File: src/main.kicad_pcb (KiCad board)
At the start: 4 copper layers, 54 parts, among them P301 CONN_01X15, P302 CONN_01X03, P501 CONN_01X07, Q501 MMBT3904, Q502 MMBT3904, U301 LM741, U302 DG444, U303 LM741, U304 LM741, U305 LM311N, U501 LM741, U502 LM741, U503 2DW232

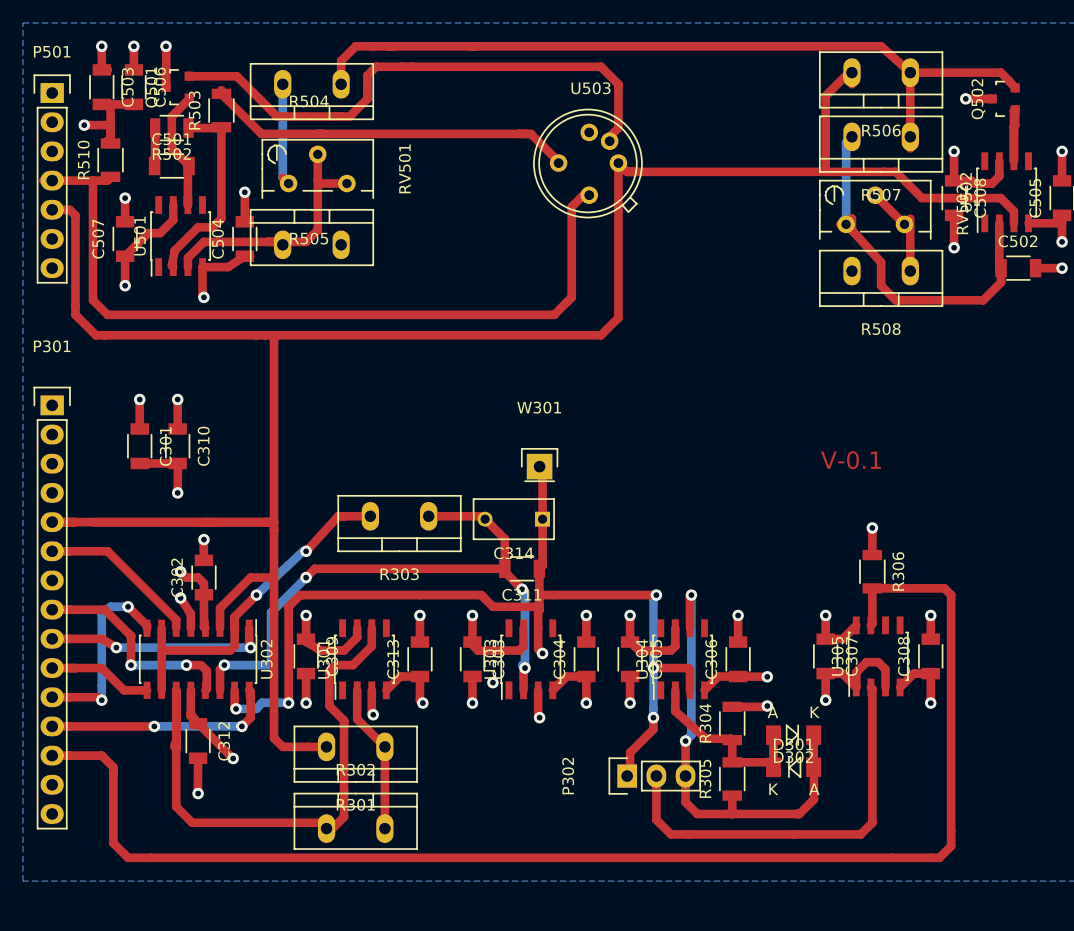
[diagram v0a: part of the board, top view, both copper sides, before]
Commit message: update
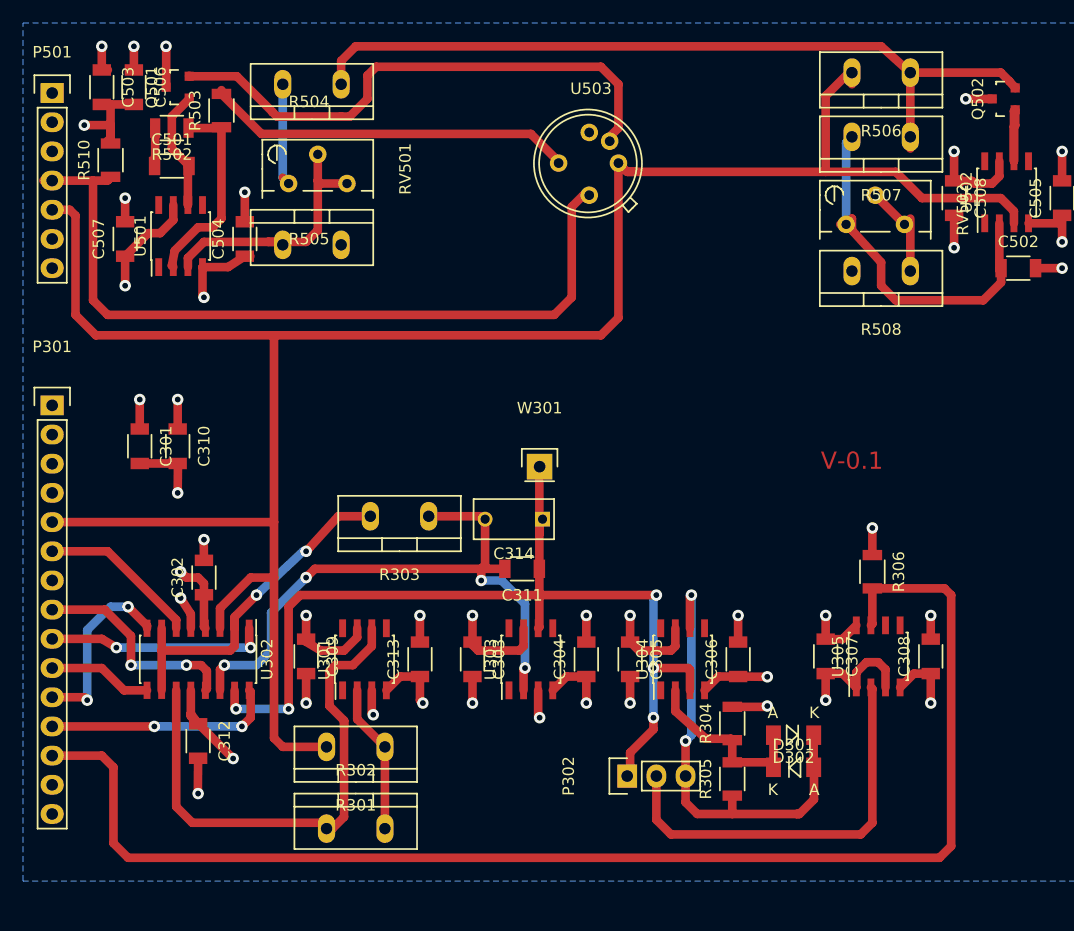
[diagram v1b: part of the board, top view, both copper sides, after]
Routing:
- net REF: track 210.8 -> 189.7 mm
- net Net-(R302-Pad1): track 51.3 -> 45.8 mm
- net Net-(C311-Pad1): track 87.7 -> 86.3 mm, vias 6 -> 5
- net Net-(Q502-Pad2): track 72.4 -> 71.0 mm
- net Net-(R503-Pad2): track 33.1 -> 32.2 mm
- net IN_CTL: track 16.9 -> 16.2 mm
- net Net-(Q501-Pad2): track 48.9 -> 48.4 mm
- net Net-(D301-Pad2): track 41.3 -> 40.8 mm
- net REF_SUB_CTL: track 9.82 -> 9.31 mm
- net (no net): vias 1 -> 0
